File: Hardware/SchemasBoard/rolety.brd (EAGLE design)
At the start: 49 x 25.9 mm, 30 parts, among them IC1 LNK302, IC3 MC33269ST-3.3T3, K1 FRS1B, K2 FRS1B, T1 BC846, T2 BC846

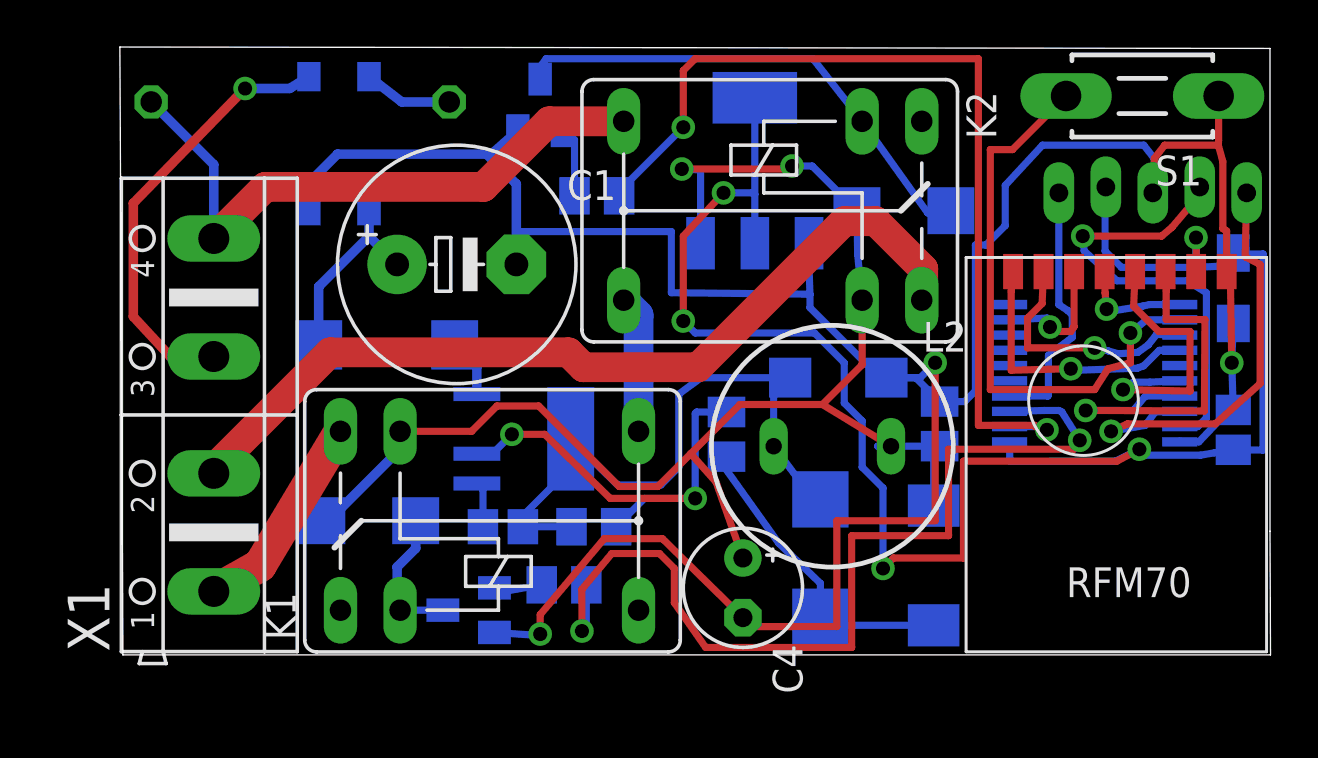
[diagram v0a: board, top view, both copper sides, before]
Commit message: a
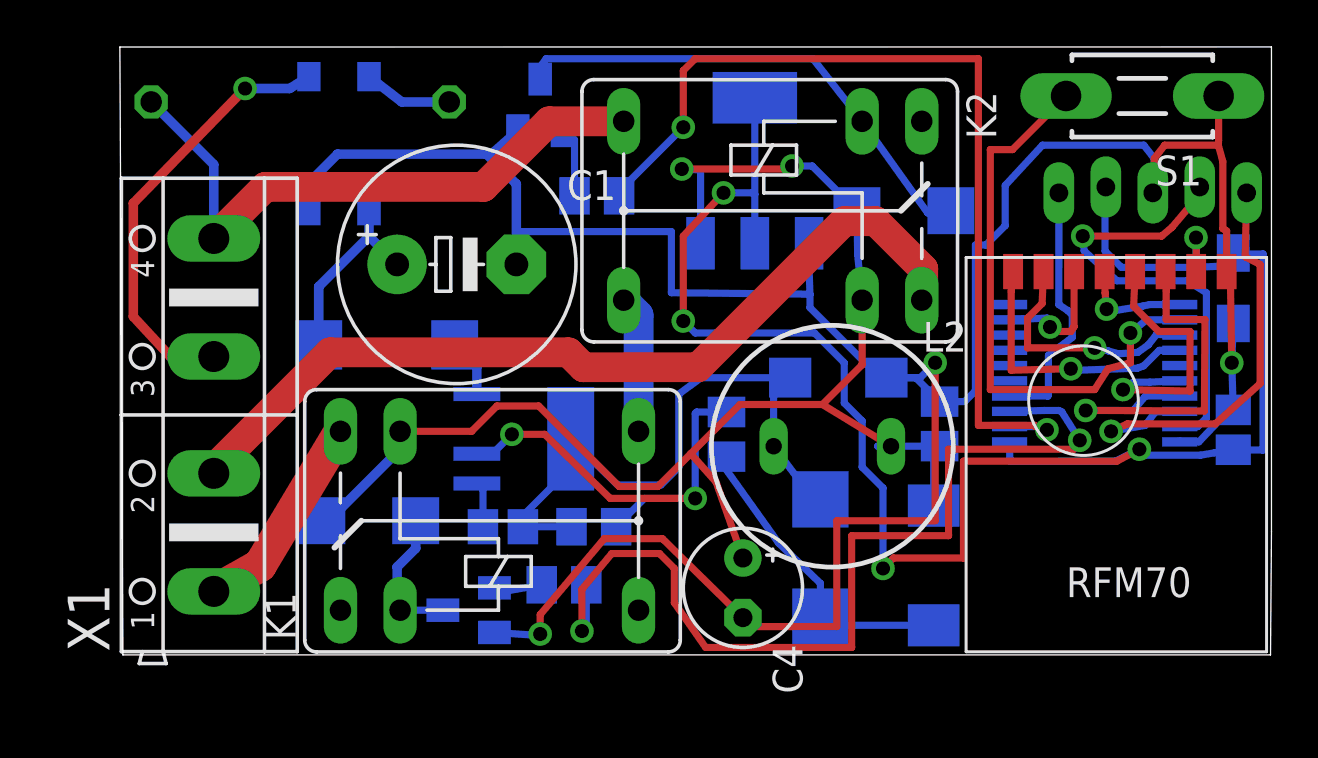
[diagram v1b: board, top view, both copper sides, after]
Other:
- board size 49 x 25.9 mm -> 49.1 x 25.9 mm
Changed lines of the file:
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@@
 <layer number="17" name="Pads" color="2" fill="1" visible="yes" active="yes"/>
 <layer number="18" name="Vias" color="2" fill="1" visible="yes" active="yes"/>
-<layer number="19" name="Unrouted" color="6" fill="1" visible="no" active="yes"/>
-<layer number="20" name="Dimension" color="15" fill="1" visible="no" active="yes"/>
-<layer number="21" name="tPlace" color="15" fill="1" visible="no" active="yes"/>
-<layer number="22" name="bPlace" color="11" fill="1" visible="no" active="yes"/>
-<layer number="23" name="tOrigins" color="15" fill="1" visible="no" active="yes"/>
-<layer number="24" name="bOrigins" color="15" fill="1" visible="no" active="yes"/>
-<layer number="25" name="tNames" color="7" fill="1" visible="no" active="yes"/>
-<layer number="26" name="bNames" color="7" fill="1" visible="no" active="yes"/>
-<layer number="27" name="tValues" color="7" fill="1" visible="no" active="yes"/>
-<layer number="28" name="bValues" color="7" fill="1" visible="no" active="yes"/>
-<layer number="29" name="tStop" color="7" fill="3" visible="no" active="yes"/>
-<layer number="30" name="bStop" color="7" fill="6" visible="no" active="yes"/>
-<layer number="31" name="tCream" color="7" fill="4" visible="no" active="yes"/>
-<layer number="32" name="bCream" color="7" fill="5" visible="no" active="yes"/>
-<layer number="33" name="tFinish" color="6" fill="3" visible="no" active="yes"/>
-<layer number="34" name="bFinish" color="6" fill="6" visible="no" active="yes"/>
-<layer number="35" name="tGlue" color="7" fill="4" visible="no" active="yes"/>
-<layer number="36" name="bGlue" color="7" fill="5" visible="no" active="yes"/>
-<layer number="37" name="tTest" color="7" fill="1" visible="no" active="yes"/>
-<layer number="38" name="bTest" color="7" fill="1" visible="no" active="yes"/>
-<layer number="39" name="tKeepout" color="4" fill="11" visible="no" active="yes"/>
-<layer number="40" name="bKeepout" color="1" fill="11" visible="no" active="yes"/>
-<layer number="41" name="tRestrict" color="4" fill="10" visible="no" active="yes"/>
-<layer number="42" name="bRestrict" color="1" fill="10" visible="no" active="yes"/>
-<layer number="43" name="vRestrict" color="2" fill="10" visible="no" active="yes"/>
-<layer number="44" name="Drills" color="7" fill="1" visible="no" active="yes"/>
-<layer number="45" name="Holes" color="7" fill="1" visible="no" active="yes"/>
-<layer number="46" name="Milling" color="3" fill="1" visible="no" active="yes"/>
-<layer number="47" name="Measures" color="7" fill="1" visible="no" active="yes"/>
-<layer number="48" name="Document" color="7" fill="1" visible="no" active="yes"/>
-<layer number="49" name="Reference" color="7" fill="1" visible="no" active="yes"/>
+<layer number="19" name="Unrouted" color="6" fill="1" visible="yes" active="yes"/>
+<layer number="20" name="Dimension" color="15" fill="1" visible="yes" active="yes"/>
+<layer number="21" name="tPlace" color="15" fill="1" visible="yes" active="yes"/>
+<layer number="22" name="bPlace" color="11" fill="1" visible="yes" active="yes"/>
+<layer number="23" name="tOrigins" color="15" fill="1" visible="yes" active="yes"/>
+<layer number="24" name="bOrigins" color="15" fill="1" visible="yes" active="yes"/>
+<layer number="25" name="tNames" color="7" fill="1" visible="yes" active="yes"/>
+<layer number="26" name="bNames" color="7" fill="1" visible="yes" active="yes"/>
+<layer number="27" name="tValues" color="7" fill="1" visible="yes" active="yes"/>
+<layer number="28" name="bValues" color="7" fill="1" visible="yes" active="yes"/>
+<layer number="29" name="tStop" color="7" fill="3" visible="yes" active="yes"/>
+<layer number="30" name="bStop" color="7" fill="6" visible="yes" active="yes"/>
+<layer number="31" name="tCream" color="7" fill="4" visible="yes" active="yes"/>
+<layer number="32" name="bCream" color="7" fill="5" visible="yes" active="yes"/>
+<layer number="33" name="tFinish" color="6" fill="3" visible="yes" active="yes"/>
+<layer number="34" name="bFinish" color="6" fill="6" visible="yes" active="yes"/>
+<layer number="35" name="tGlue" color="7" fill="4" visible="yes" active="yes"/>
+<layer number="36" name="bGlue" color="7" fill="5" visible="yes" active="yes"/>
+<layer number="37" name="tTest" color="7" fill="1" visible="yes" active="yes"/>
+<layer number="38" name="bTest" color="7" fill="1" visible="yes" active="yes"/>
+<layer number="39" name="tKeepout" color="4" fill="11" visible="yes" active="yes"/>
+<layer number="40" name="bKeepout" color="1" fill="11" visible="yes" active="yes"/>
+<layer number="41" name="tRestrict" color="4" fill="10" visible="yes" active="yes"/>
+<layer number="42" name="bRestrict" color="1" fill="10" visible="yes" active="yes"/>
+<layer number="43" name="vRestrict" color="2" fill="10" visible="yes" active="yes"/>
+<layer number="44" name="Drills" color="7" fill="1" visible="yes" active="yes"/>
+<layer number="45" name="Holes" color="7" fill="1" visible="yes" active="yes"/>
+<layer number="46" name="Milling" color="3" fill="1" visible="yes" active="yes"/>
+<layer number="47" name="Measures" color="7" fill="1" visible="yes" active="yes"/>
+<layer number="48" name="Document" color="7" fill="1" visible="yes" active="yes"/>
+<layer number="49" name="Reference" color="7" fill="1" visible="yes" active="yes"/>
 <layer number="50" name="dxf" color="7" fill="1" visible="no" active="no"/>
-<layer number="51" name="tDocu" color="7" fill="1" visible="no" active="yes"/>
-<layer number="52" name="bDocu" color="7" fill="1" visible="no" active="yes"/>
+<layer number="51" name="tDocu" color="7" fill="1" visible="yes" active="yes"/>
+<layer number="52" name="bDocu" color="7" fill="1" visible="yes" active="yes"/>
 <layer number="91" name="Nets" color="2" fill="1" visible="no" active="no"/>
 <layer number="92" name="Busses" color="1" fill="1" visible="no" active="no"/>
@@
 <plain>
 <wire x1="-1.143" y1="0" x2="47.752" y2="0" width="0" layer="20"/>
-<wire x1="47.752" y1="0" x2="47.729" y2="5.2705" width="0" layer="20"/>
-<wire x1="47.729" y1="5.2705" x2="47.729" y2="25.838" width="0" layer="20"/>
-<wire x1="47.729" y1="25.838" x2="-1.27" y2="25.898" width="0" layer="20"/>
+<wire x1="47.752" y1="0" x2="47.7925" y2="5.2705" width="0" layer="20"/>
+<wire x1="47.7925" y1="5.2705" x2="47.7925" y2="25.9015" width="0" layer="20"/>
+<wire x1="47.7925" y1="25.9015" x2="-1.27" y2="25.898" width="0" layer="20"/>
 <wire x1="-1.27" y1="25.898" x2="-1.143" y2="0" width="0" layer="20"/>
 </plain>
@@
 </signal>
 </signals>
-<errors>
-</errors>
 </board>
 </drawing>

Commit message: Refactoring
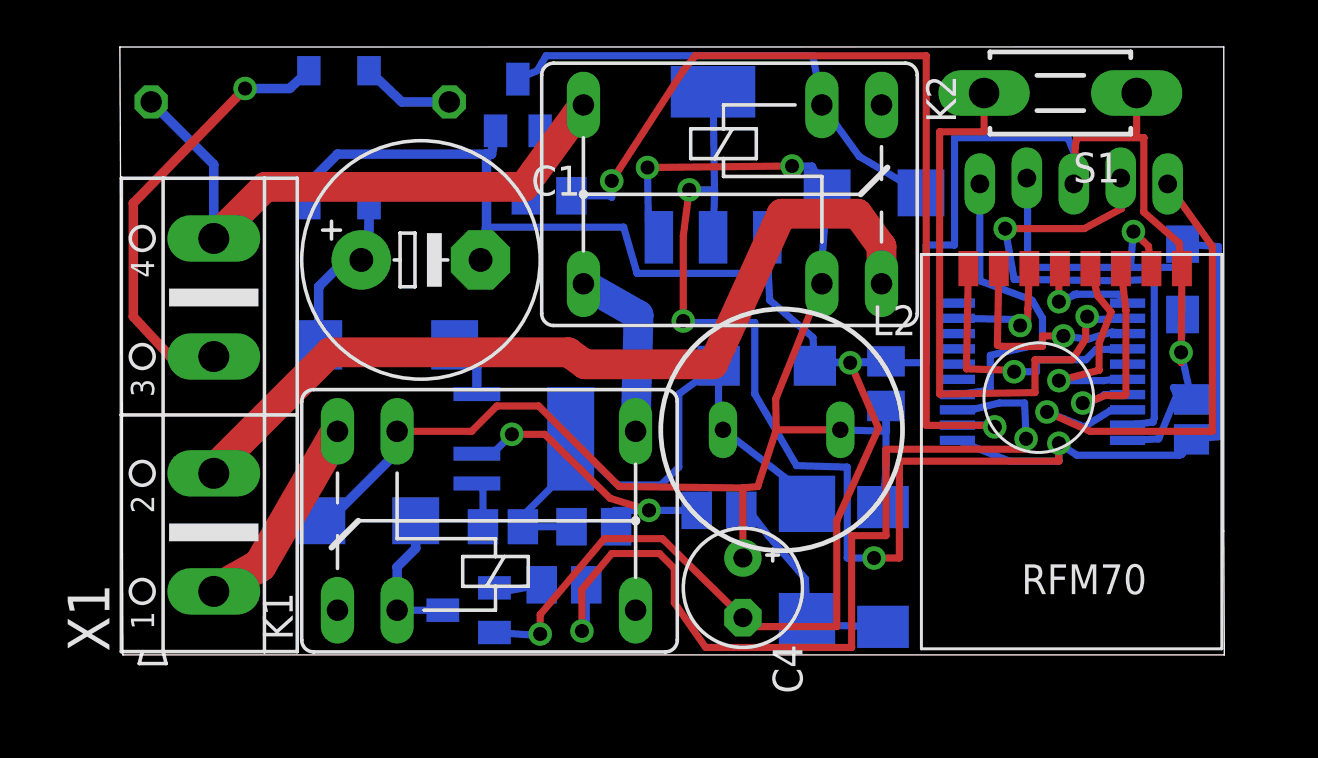
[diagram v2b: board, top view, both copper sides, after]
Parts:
- moved S1 3.49 mm to (38.8, 23.9)
- moved U$3 3.39 mm to (39.4, 20.1)
- moved R3 3.25 mm to (24.3, 6.16), turned to 0 degrees
- moved D3 3.09 mm to (26.3, 12.3)
- moved R7 2.86 mm to (31.4, 11.6)
- moved L2 2.27 mm to (26.9, 9.59)
- moved U$2 2.22 mm to (38.0, 12.1)
- moved C6 2.19 mm to (44.0, 16.0)
- moved D4 2.16 mm to (31.2, 3.75)
- moved R6 2.03 mm to (17.0, 19.6)
- moved U$1 1.91 mm to (43.9, 2.16)
- moved K2 1.85 mm to (28.6, 19.6)
- moved C5 1.83 mm to (44.4, 10.0)
- moved IC3 1.80 mm to (24.0, 20.9)
- moved C1 1.54 mm to (11.6, 16.8)
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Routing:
- net N$16: track 16.9 -> 9.29 mm
- net N$11: track 20.3 -> 13.7 mm
- net N$9: track 13.6 -> 9.17 mm
- net GND: track 121.7 -> 118.0 mm
- net N$19: track 18.8 -> 22.1 mm
- net N$20: track 12.3 -> 9.44 mm
- net N$18: track 19.2 -> 21.8 mm
- net N$25: track 11.1 -> 13.6 mm
- net N$27: track 62.3 -> 60.1 mm
- net N$26: track 5.85 -> 7.66 mm
- net N$13: track 27.5 -> 25.8 mm
- net N$35: track 40.8 -> 39.4 mm
- net N$5: track 24.5 -> 25.6 mm
- net N$36: track 26.5 -> 25.4 mm
- net N$12: track 10.3 -> 9.32 mm
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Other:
- board size 49.1 x 25.9 mm -> 47.1 x 25.9 mm
